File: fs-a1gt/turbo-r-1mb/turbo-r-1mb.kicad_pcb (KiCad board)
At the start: 2 copper layers, 71.5 x 27 mm, 19 parts, among them U1 220-1-20-003, U2 220-1-20-003, U3 KM44C1000, U4 SN74LS670D, U5 CD74HCT367M96, U6 CD74HCT30M96, U7 SN74HCT32DR, U8 KM44C1000

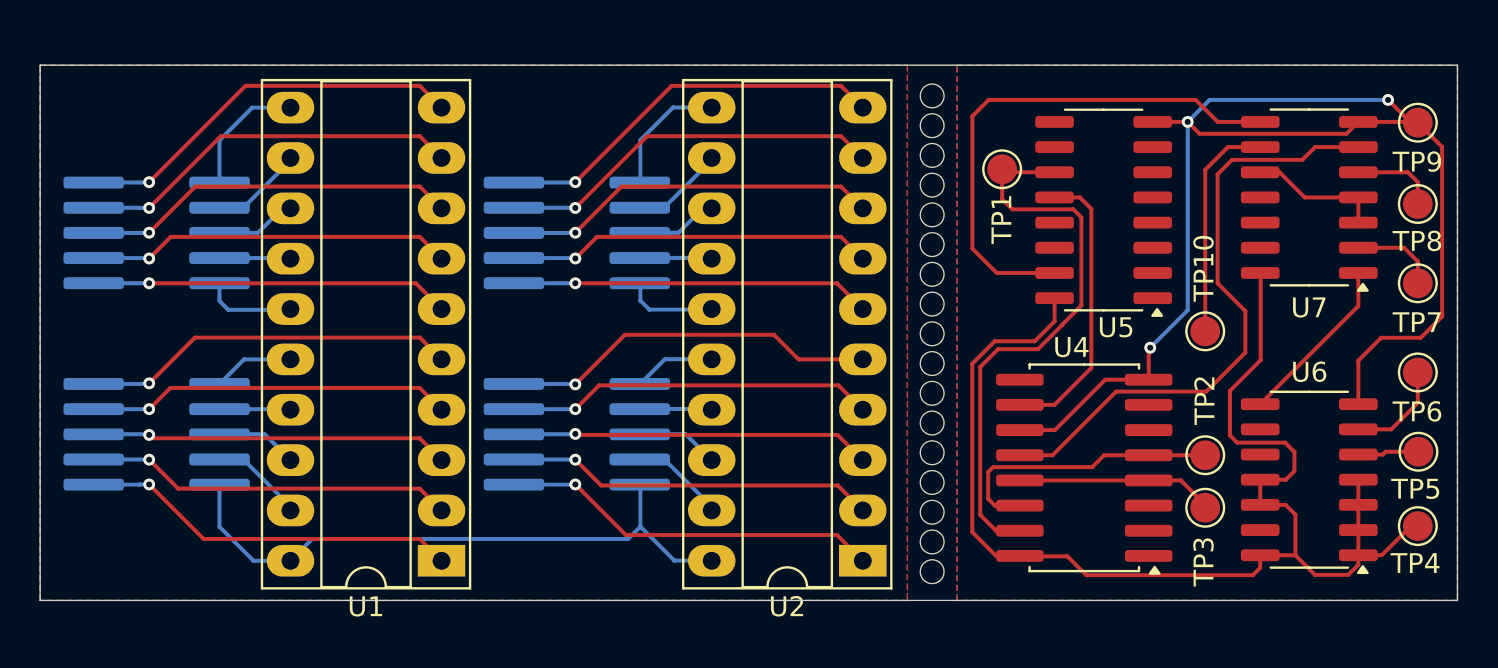
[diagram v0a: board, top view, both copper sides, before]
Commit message: PCB ready for ordering
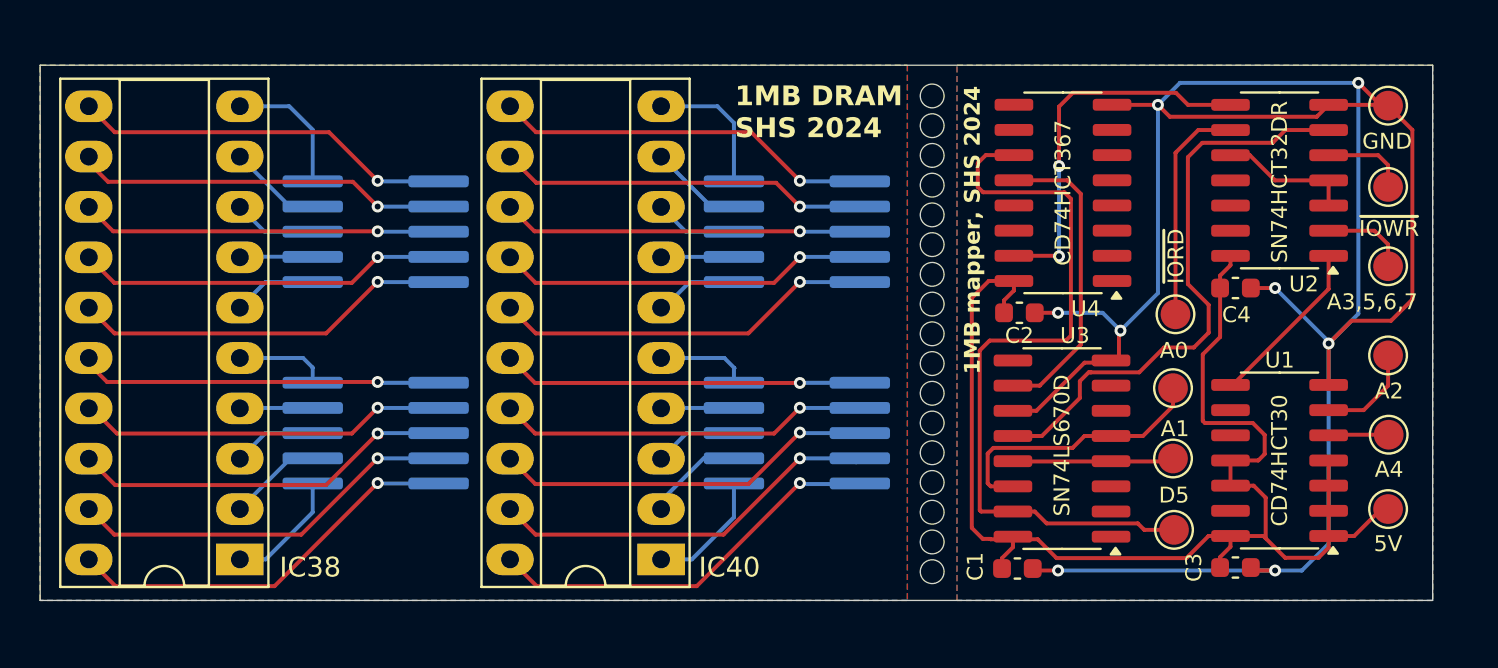
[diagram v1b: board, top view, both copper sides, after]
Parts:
- added C1: 100nF, Capacitor_SMD:C_0603_1608Metric, F.Cu at (158.3, 110.6)
- added C2: 100nF, Capacitor_SMD:C_0603_1608Metric, F.Cu at (158.4, 97.7)
- added C3: 100nF, Capacitor_SMD:C_0603_1608Metric, F.Cu at (169.3, 110.6)
- added C4: 100nF, Capacitor_SMD:C_0603_1608Metric, F.Cu at (169.3, 96.5)
- TP1: value D6 -> D5
- TP10: value nIORD -> ~{IORD}
- TP7: value nA[3/5/6/7] -> A3,5,6,7
- TP8: value nIOWR -> ~{IOWR}
- U1: renamed from U6; value CD74HCT30M96 -> CD74HCT30
- U3: renamed from U4; footprint Package_SO:SOIC-16W_5.3x10.2mm_P1.27mm -> Package_SO:SOIC-16_3.9x9.9mm_P1.27mm
- U4: renamed from U5; value CD74HCT367M96 -> CD74HCT367
- moved TP1 20.2 mm to (166.2, 108.7)
- moved IC2 11.1 mm to (147.2, 98.7)
- moved IC1 11.1 mm to (125.9, 98.7)
- moved IC40 10.2 mm to (140.3, 110.2)
- moved IC38 10.2 mm to (119.1, 110.2)
- moved TP2 3.75 mm to (166.2, 101.5)
- moved TP3 2.97 mm to (166.2, 105.1)
- moved U4 2.23 mm to (160.6, 91.7)
- moved U1 1.79 mm to (171.5, 105.2)
- moved TP10 1.73 mm to (166.3, 97.8)
- moved TP4 1.73 mm to (177.0, 107.6)
- moved TP5 1.73 mm to (177.0, 103.9)
- moved TP6 1.73 mm to (177.0, 99.9)
- moved TP7 1.73 mm to (177.0, 95.4)
- moved TP8 1.73 mm to (177.0, 91.4)
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- renumbered U3 to IC1, U8 to IC2, U1 to IC38, U2 to IC40, U7 to U2
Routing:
- net GND: track 65.4 -> 115.2 mm, vias 3 -> 8
- net /DQ2A: track 4.12 -> 19.5 mm, vias 0 -> 1
- net /DQ2B: track 4.12 -> 19.3 mm, vias 0 -> 1
- net /DQ3B: track 4.76 -> 20.0 mm, vias 0 -> 1
- net /A7A: track 3.59 -> 18.7 mm, vias 0 -> 1
- net /A7B: track 3.59 -> 18.7 mm, vias 0 -> 1
- net /~{CASA}: track 3.59 -> 18.7 mm, vias 0 -> 1
- net /~{CASB}: track 3.59 -> 18.7 mm, vias 0 -> 1
- net /DQ3A: track 4.76 -> 19.8 mm, vias 0 -> 1
- net /~{RASB}: track 18.6 -> 3.73 mm, vias 1 -> 0
- net /A1A: track 18.5 -> 3.59 mm, vias 1 -> 0
- net /A1B: track 18.5 -> 3.73 mm, vias 1 -> 0
- net /~{RASA}: track 18.4 -> 3.73 mm, vias 1 -> 0
- net /A8A: track 4.67 -> 19.3 mm, vias 0 -> 1
- net /A8B: track 4.67 -> 19.3 mm, vias 0 -> 1
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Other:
- board size 71.5 x 27 mm -> 70.2 x 27 mm
- board text added: "1MB DRAM SHS 2024"
- board text added: "1MB mapper, SHS 2024"
